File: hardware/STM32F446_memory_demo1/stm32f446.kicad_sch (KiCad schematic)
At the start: 28 parts, among them U301 STM32F446ZCT6, Y301 16MHz

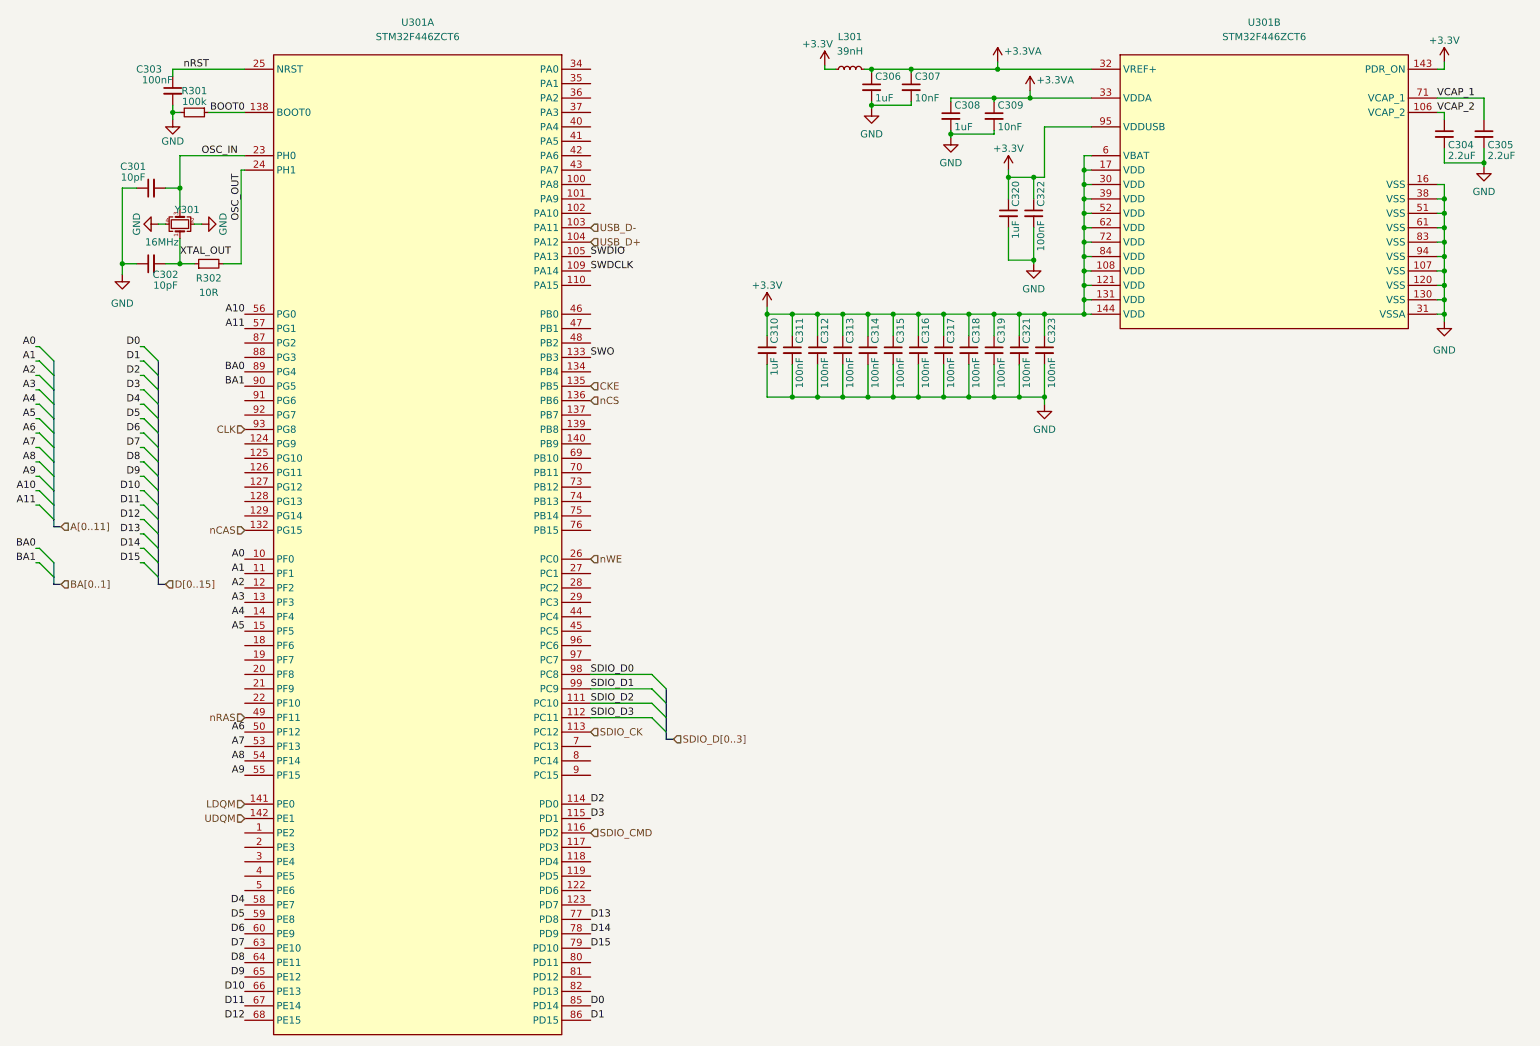
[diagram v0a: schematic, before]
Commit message: added a lot of stuff a long time ago :S
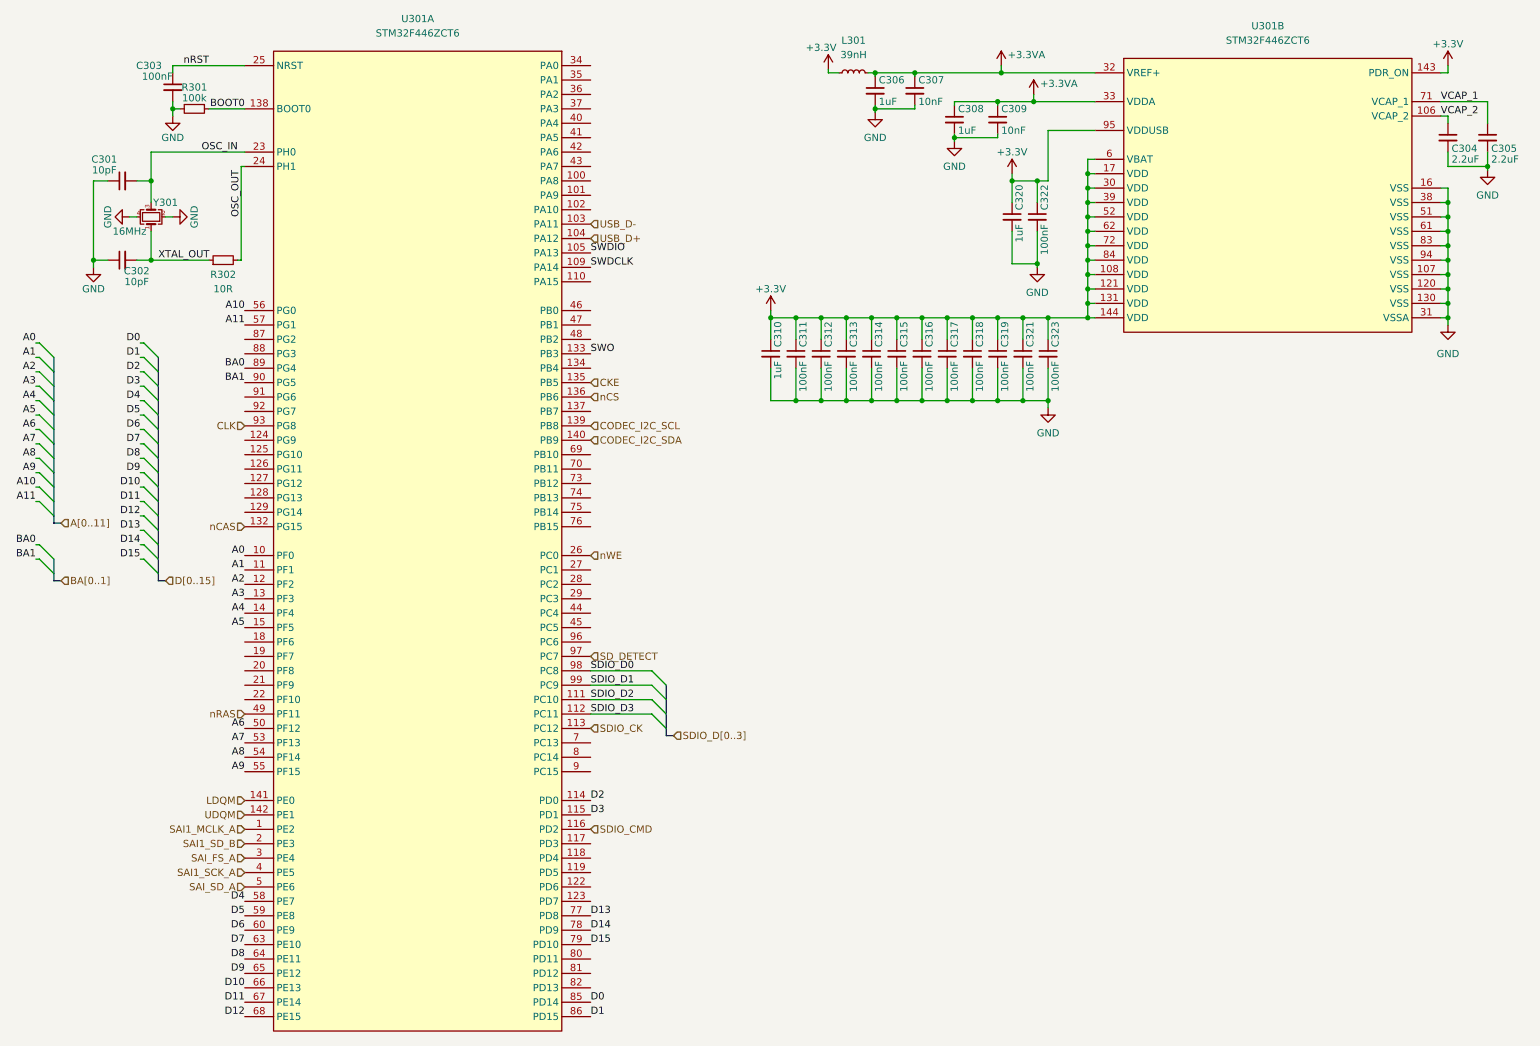
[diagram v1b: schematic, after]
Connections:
- net SAI1_MCLK_A: now reaches U301.1 (PE2)
- net CODEC_I2C_SCL: now reaches U301.139 (PB8)
- net CODEC_I2C_SDA: now reaches U301.140 (PB9)
- net SAI1_SD_B: now reaches U301.2 (PE3)
- net SAI_FS_A: now reaches U301.3 (PE4)
- net SAI1_SCK_A: now reaches U301.4 (PE5)
- net SAI_SD_A: now reaches U301.5 (PE6)
- net SD_DETECT: now reaches U301.97 (PC7)
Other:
- moved on the sheet: C301, C302, C303, C304, C305, C306, C307, C308, C309, C310, C311, C312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
